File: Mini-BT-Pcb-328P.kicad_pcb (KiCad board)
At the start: 2 copper layers, 55 x 35 mm, 51 parts, among them J1 Analog IN, J2 USB_B_Micro, J5 ANT, J6 Booster, P1 MYSX_2.6, Q1 FDN338P, Q2 FDN337N, SW2 Reset, SW3 SW_Reed, U1 ME2188C33, U2 ATSHA204A, U3 AMS1117-3.3, U4 ATmega328P-AU, U5 NRF24L01, U6 NRF24L01, U7 RFM69HW

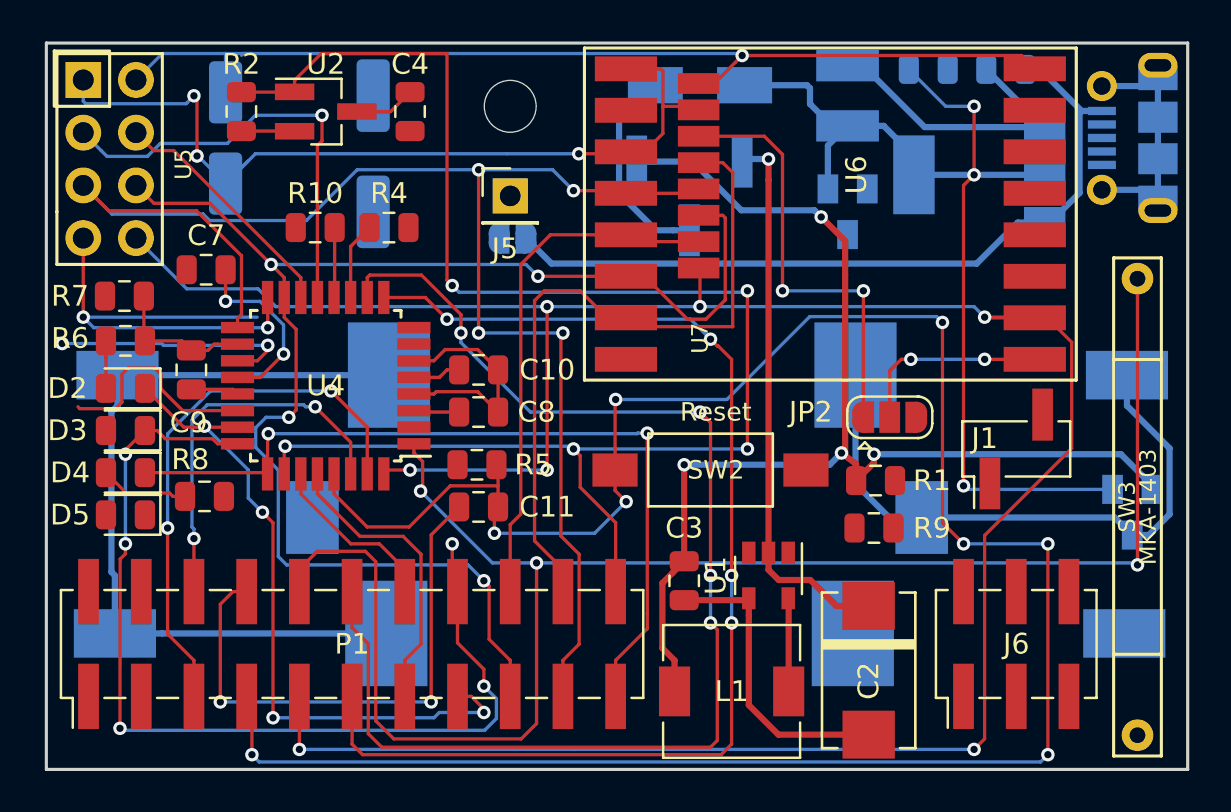
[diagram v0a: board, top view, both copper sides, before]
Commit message: routing test 2
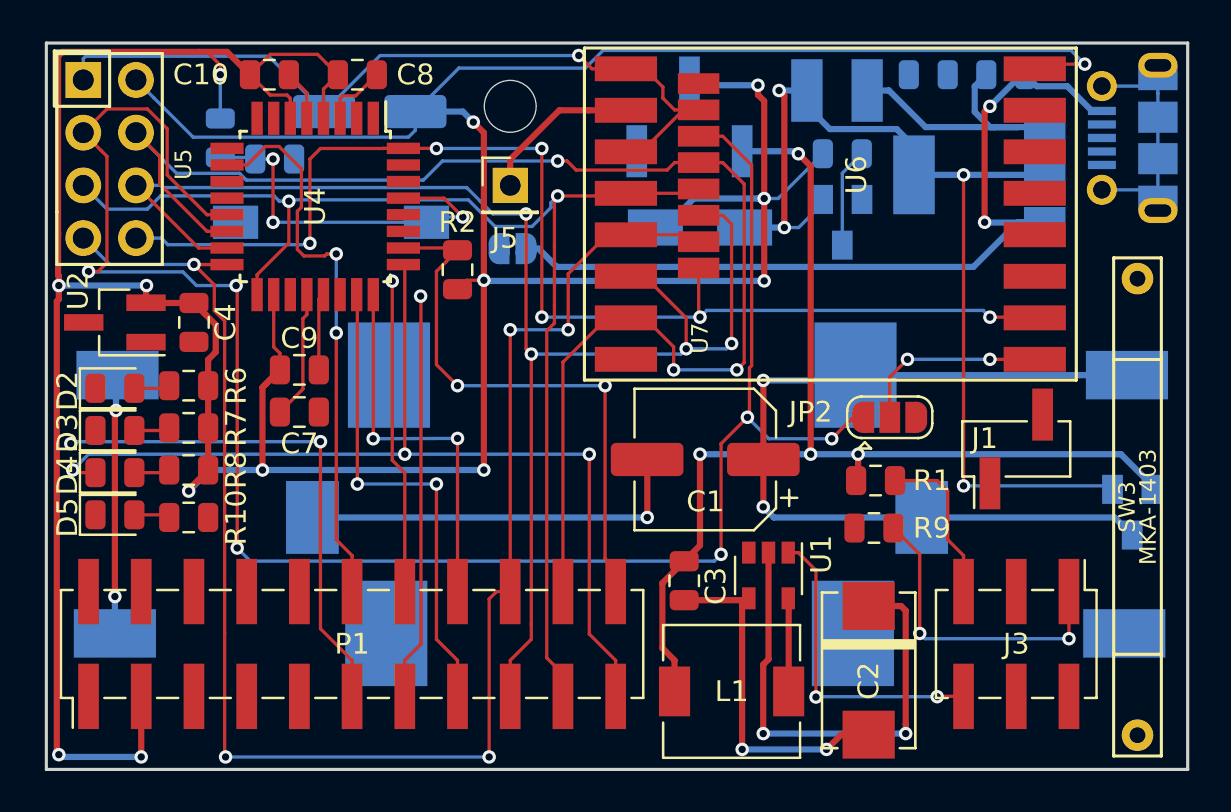
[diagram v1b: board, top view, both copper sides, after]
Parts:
- removed J6: Booster, Connector_PinHeader_2.54mm:PinHeader_2x03_P2.54mm_Vertical_SMD
- added J3: Booster CE, Connector_PinHeader_2.54mm:PinHeader_2x03_P2.54mm_Vertical_SMD, F.Cu at (178.8, 102.4)
- C1: moved to F.Cu
- C11, R4, R5, SW2: moved to B.Cu
- moved R4 22.1 mm to (170.4, 78.7), turned to 180 degrees
- moved SW2 21.8 mm to (145.8, 82.0), turned to 0 degrees
- moved C1 21.8 mm to (163.8, 93.5), turned to 180 degrees
- moved R5 20.0 mm to (140.5, 78.0), turned to 90 degrees
- moved C11 19.4 mm to (143.1, 79.0), turned to 0 degrees
- moved C10 17.4 mm to (142.8, 74.9), turned to 180 degrees
- moved C8 17.3 mm to (147.1, 74.9), turned to 180 degrees
- moved R10 15.2 mm to (138.9, 96.3)
- moved C4 14.5 mm to (139.2, 86.9), turned to 90 degrees
- moved U2 14.4 mm to (135.4, 86.9), turned to 180 degrees
- moved R2 12.9 mm to (151.9, 84.3)
- moved U4 8.65 mm to (145.0, 81.3), turned to 270 degrees
- moved C7 8.20 mm to (144.3, 91.2), turned to 0 degrees
- moved R7 7.06 mm to (138.9, 91.9)
- moved C12 7.06 mm to (147.7, 76.7), turned to 180 degrees
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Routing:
- net VCC: track 81.3 -> 218.2 mm, vias 1 -> 14
- net RESET: track 110.6 -> 18.2 mm, vias 8 -> 3
- net D3: track 81.5 -> 0.00 mm, vias 3 -> 0
- net D2: track 125.1 -> 58.6 mm, vias 7 -> 6
- net D9: track 42.7 -> 91.3 mm, vias 3 -> 6
- net A3: track 75.7 -> 27.3 mm, vias 5 -> 2
- net D6: track 62.2 -> 27.0 mm, vias 4 -> 2
- net D5: track 57.5 -> 25.0 mm, vias 4 -> 2
- net MISO: track 48.0 -> 78.6 mm, vias 2 -> 5
- net A1: track 47.3 -> 18.4 mm, vias 5 -> 2
- net D1-TXD: track 26.6 -> 0.00 mm, vias 2 -> 0
- net DTR: track 26.3 -> 0.00 mm, vias 2 -> 0
- net Net-(BT2-Pad2): track 38.8 -> 12.5 mm, vias 0 -> 2
- net NSS: track 46.1 -> 69.8 mm, vias 0 -> 3
- net D0-RXD: track 18.5 -> 0.00 mm, vias 2 -> 0
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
